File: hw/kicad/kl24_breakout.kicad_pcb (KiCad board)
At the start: 2 copper layers, 36.1 x 20.8 mm, 53 parts, among them J1 USB-micro-ab, P1 TST, P10 TST, P11 TST, P12 TST, P13 TST, P14 TST, P15 TST, P16 TST, P17 TST, P18 TST, P19 TST, P2 TST, P20 TST, P21 TST, P22 TST, P23 TST, P24 TST, P25 TST, P26 TST, P27 TST, P28 TST, P29 TST, P3 TST, P30 TST, P31 TST, P32 TST, P33 USB_V, P34 USB_GND, P35 SWD_VCC, P36 SWDIO, P37 SWCLK, P38 NRESET, P39 SWD_GND, P4 TST, P5 TST, P6 TST, P7 TST, P8 TST, P9 TST, U1 MKL24Z64VFM4, U2 LP3985, X1 CRYSTAL

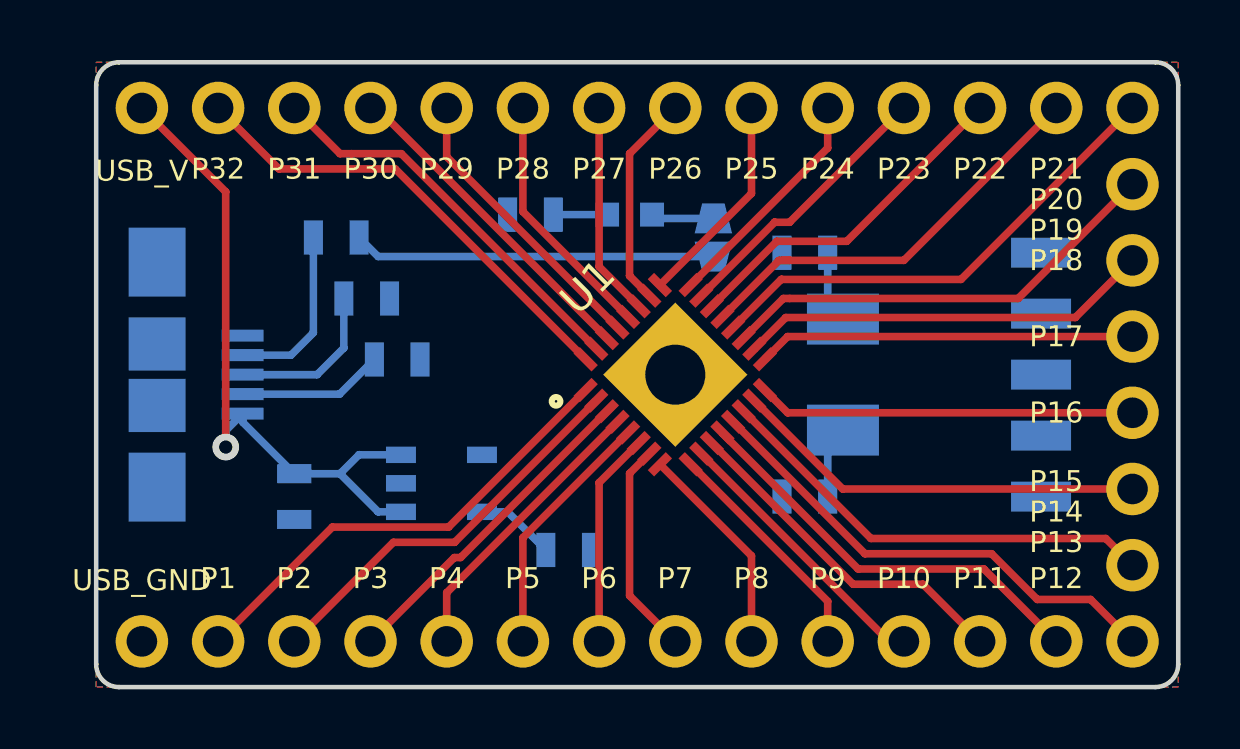
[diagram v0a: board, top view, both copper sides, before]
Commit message: tweak pcb
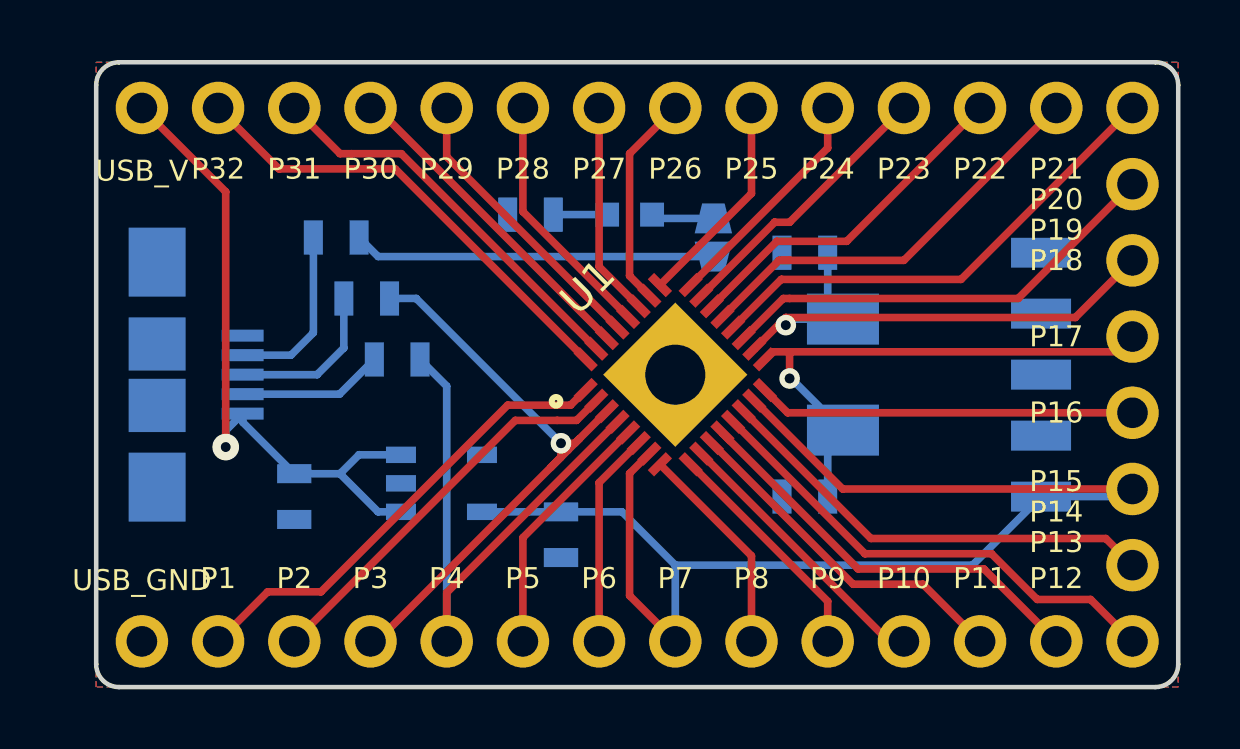
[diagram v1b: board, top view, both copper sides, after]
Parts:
- moved C1 8.13 mm to (133.9, 75.2)
- moved C2 8.13 mm to (133.9, 67.1)
- moved C4 0.57 mm to (125.7, 76.5), turned to 270 degrees
- turned X1 to 270 degrees
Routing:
- net 15: track 23.6 -> 47.0 mm
- net 3: track 11.1 -> 21.0 mm, vias 0 -> 1
- net 4: track 9.67 -> 19.4 mm
- net 17: track 15.0 -> 18.4 mm, vias 0 -> 1
- net 18: track 16.2 -> 18.5 mm, vias 0 -> 1
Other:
- net class Default: via_dia 0.889 -> 0.6858; via_drill 0.635 -> 0.3302
- rule via_min_drill: 0.508 -> 0.3302
- rule via_min_size: 0.889 -> 0.6858
